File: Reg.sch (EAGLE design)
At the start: 25 parts, among them Q1 NPN, Q2 NPN, Q3 PNP, Q4 NPN, Q5 NPN, Q6 NPN, Q8 PNP

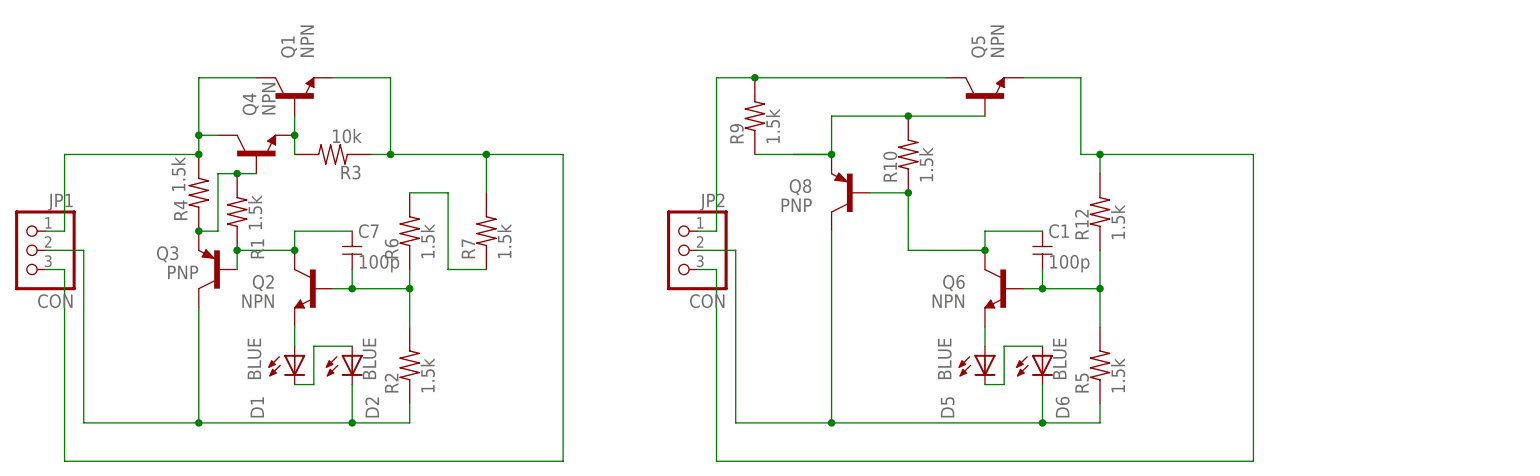
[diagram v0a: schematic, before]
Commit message: OPA ver
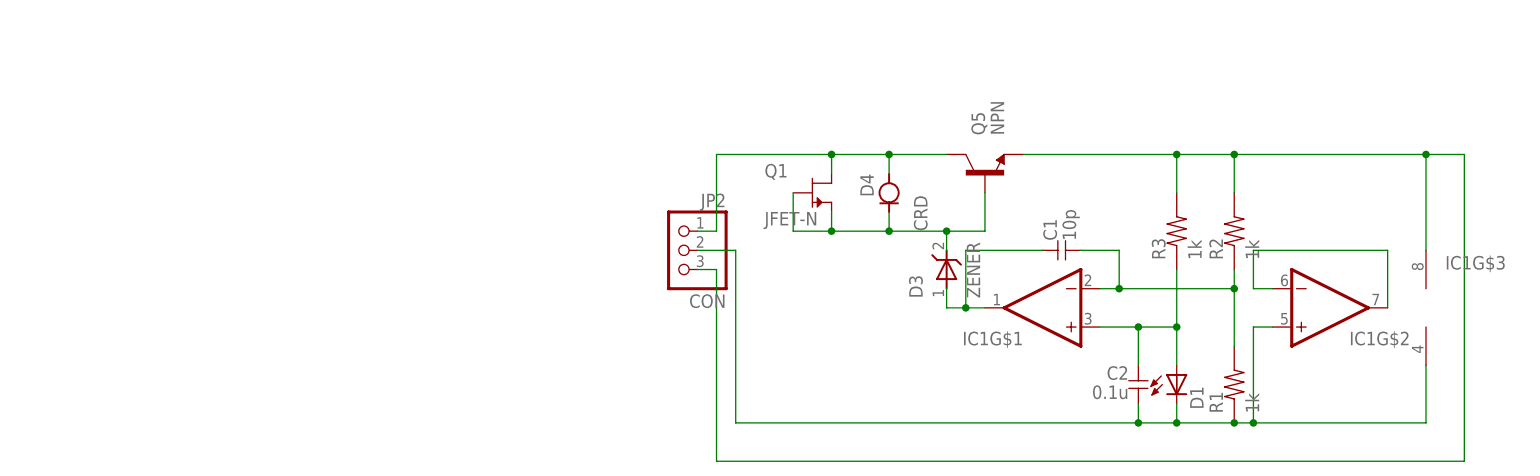
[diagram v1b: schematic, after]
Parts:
- removed C7: 100p, my_rcl:C-1608
- removed D2, D5, D6: BLUE, my_rcl:LED-SMD1608
- removed JP1: CON, pinhead:PINHD-1X3
- removed Q2, Q4, Q6: NPN, my_ic:NPN2SC3325
- removed Q3, Q8: PNP, my_ic:PNP2SA1313
- removed R10, R12, R4, R5, R6, R7, R9: 1.5k, my_rcl:R-1608
- added C2: 0.1u, my_rcl:C-2012
- added D3: ZENER, my_rcl:ZENER-SMD
- added D4: CRD, my_rcl:CRD-SMD
- added IC1: (no value), my_ic:OPA-2-SOP
- C1: value 100p -> 10p
- D1: value BLUE -> (none); device my_rcl:LED-SMD1608 -> my_rcl:LED-SMD2012
- JP2: device pinhead:PINHD-1X3 -> my_connector:SW-1X3
- Q1: value NPN -> JFET-N; device my_ic:NPN2SC3422-2 -> my_ic:JFET-N
- Q5: device my_ic:NPN-SOT223 -> my_ic:NPN2SC3422-2
- R1, R2: value 1.5k -> 1k
- R3: value 10k -> 1k
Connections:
- removed net GND: D2.K, JP1.2, Q3.C, R2.1
- removed net IN: JP1.1, Q1.C, Q4.C, R4.2
- removed net N$10: C7.1, Q2.C, Q3.B, R1.1
- removed net N$12: C1.1, Q6.C, Q8.B, R10.1
- removed net N$13: C1.2, Q6.B, R12.1, R5.2
- removed net N$16: Q5.B, Q8.E, R10.2, R9.1
- removed net N$6: Q1.B, Q4.E, R3.2
- removed net N$8: D5.K, D6.A
- removed net N$9: D5.A, Q6.E
- removed net OUT: JP1.3, Q1.E, R3.1, R7.2
- net GND1: now also C2.2, D1.K, IC1G$2.+IN, IC1G$3.V-, R1.1; no longer D6.K, Q8.C, R5.1
- net IN1: now also D4.A, Q1.D; no longer R9.2
- net N$1: now also C2.1, D1.A, IC1G$1.+IN, R3.1; no longer Q3.E, Q4.B, R1.2, R4.1
- net N$2: now also D3.C, D4.K, Q1.G, Q1.S, Q5.B; no longer D1.K, D2.A
- net N$3: now also C1.2, IC1G$1.-IN, R1.2, R2.1; no longer C7.2, Q2.B, R2.2, R6.1
- net N$4: now also C1.1, D3.A, IC1G$1.OUT; no longer D1.A, Q2.E
- net N$5: now also IC1G$2.-IN, IC1G$2.OUT; no longer R6.2, R7.1
- net OUT1: now also IC1G$3.V+, R2.2, R3.2; no longer R12.2
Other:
- moved on the sheet: C1, D1, Q5, R1, R2, R3
